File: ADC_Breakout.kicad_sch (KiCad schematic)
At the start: 36 parts, among them J0 Conn_01x06, J10 Conn_01x02, J11 Conn_01x02, J12 Conn_01x02, J13 Conn_01x02, J2 Digital Power, J3 Clock Chooser, J4 Analog Power, J6 Conn_01x02, J7 Conn_01x02, J8 Conn_01x02, J9 Conn_01x02, SW1 SW_MEC_5E, U2 SN74AUP2G80DCUR, X1 SIT8924BA-22-33E-8.192000, Y1 Crystal_Small

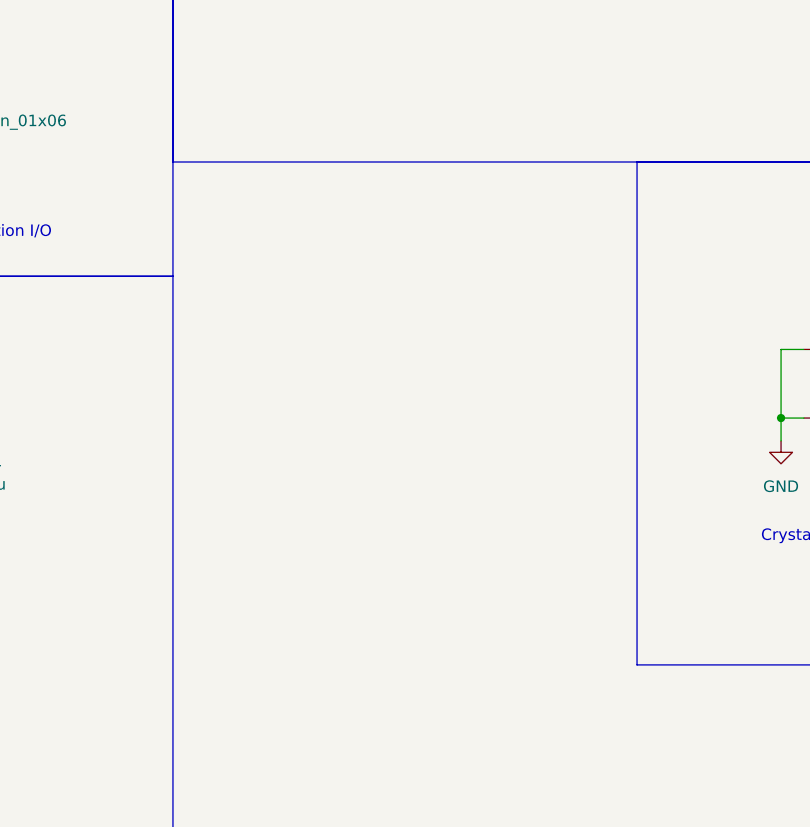
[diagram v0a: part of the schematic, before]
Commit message: Added graphics + iBOM
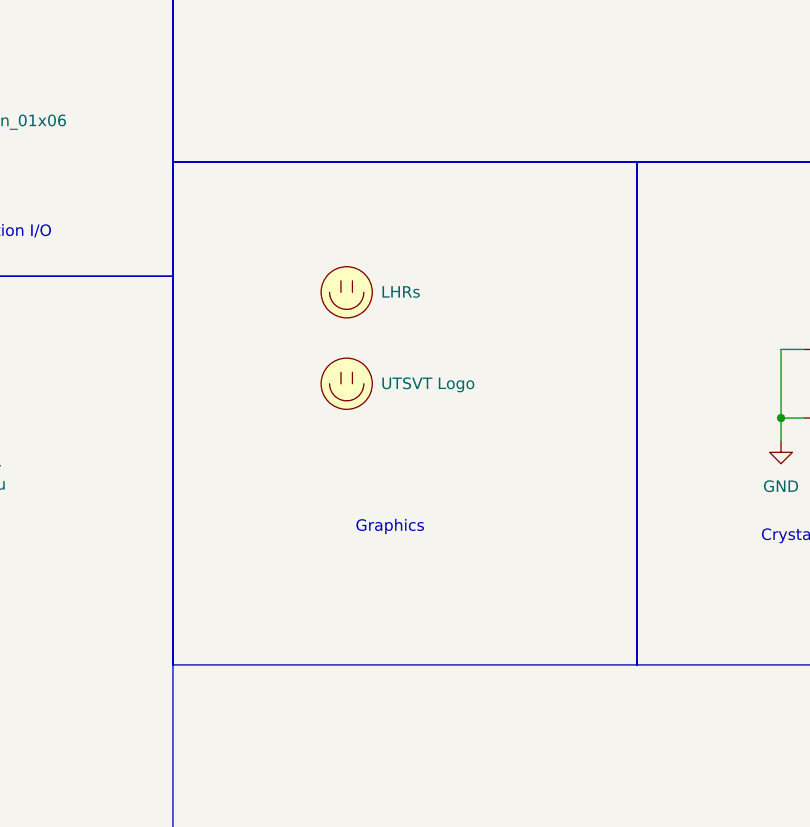
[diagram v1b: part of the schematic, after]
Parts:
- added LOGO0: LHRs, Top:LHRs_LOGO, symbol UTSVT_Misc:Logo_Placeholder
- added LOGO1: UTSVT Logo, SVT_Special:UTSVT_Logo_Symbol, symbol UTSVT_Misc:Logo_Placeholder
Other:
- note added: "Graphics"
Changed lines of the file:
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@@
 	)
 	(rectangle
+		(start 125.476 109.982)
+		(end 177.038 165.862)
+		(stroke
+			(width 0)
+			(type default)
+		)
+		(fill
+			(type none)
+		)
+	)
+	(rectangle
 		(start 11.938 122.682)
 		(end 125.476 198.12)
@@
 		)
 	)
+	(text "Graphics"
+		(exclude_from_sim no)
+		(at 149.606 150.622 0)
+		(effects
+			(font
+				(size 1.27 1.27)
+			)
+		)
+	)
 	(text "External Oscillator\nChosen from TI Development Board"
 		(exclude_from_sim no)
@@
 	)
 	(symbol
+		(lib_id "UTSVT_Misc:Logo_Placeholder")
+		(at 144.78 124.46 0)
+		(unit 1)
+		(exclude_from_sim no)
+		(in_bom yes)
+		(on_board yes)
+		(dnp no)
+		(fields_autoplaced yes)
+		(property "Reference" "LOGO0"
+			(at 144.78 120.65 0)
+			(effects
+				(font
+					(size 1.27 1.27)
+				)
+				(hide yes)
+			)
+		)
+		(property "Value" "LHRs"
+			(at 148.59 124.4599 0)
+			(effects
+				(font
+					(size 1.27 1.27)
+				)
+				(justify left)
+			)
+		)
+		(property "Footprint" "Top:LHRs_LOGO"
+			(at 144.78 122.555 0)
+			(effects
+				(font
+					(size 1.27 1.27)
+				)
+				(hide yes)
+			)
+		)
+		(property "Datasheet" ""
+			(at 144.78 122.555 0)
+			(effects
+				(font
+					(size 1.27 1.27)
+				)
+				(hide yes)
+			)
+		)
+		(property "Description" "Graph footprint placeholder"
+			(at 144.78 124.46 0)
+			(effects
+				(font
+					(size 1.27 1.27)
+				)
+				(hide yes)
+			)
+		)
+		(instances
+			(project ""
+				(path "/9e6f337e-b8cc-44e4-808a-ba1b350193a1"
+					(reference "LOGO0")
+					(unit 1)
+				)
+			)
+		)
+	)
+	(symbol
 		(lib_id "power:GND")
 		(at 236.22 52.07 0)
@@
 					(unit 1)
 				)
+			)
+		)
+	)
+	(symbol
+		(lib_id "UTSVT_Misc:Logo_Placeholder")
+		(at 144.78 134.62 0)
+		(unit 1)
+		(exclude_from_sim no)
+		(in_bom yes)
+		(on_board yes)
+		(dnp no)
+		(fields_autoplaced yes)
+		(property "Reference" "LOGO1"
+			(at 144.78 130.81 0)
+			(effects
+				(font
+					(size 1.27 1.27)
+				)
+				(hide yes)
+			)
+		)
+		(property "Value" "UTSVT Logo"
+			(at 148.59 134.6199 0)
+			(effects
+				(font
+					(size 1.27 1.27)
+				)
+				(justify left)
+			)
+		)
+		(property "Footprint" "SVT_Special:UTSVT_Logo_Symbol"
+			(at 144.78 132.715 0)
+			(effects
+				(font
+					(size 1.27 1.27)
+				)
+				(hide yes)
+			)
+		)
+		(property "Datasheet" ""
+			(at 144.78 132.715 0)
+			(effects
+				(font
+					(size 1.27 1.27)
+				)
+				(hide yes)
+			)
+		)
+		(property "Description" "Graph footprint placeholder"
+			(at 144.78 134.62 0)
+			(effects
+				(font
+					(size 1.27 1.27)
+				)
+				(hide yes)
+			)
+		)
+		(instances
+			(project "ADC_Breakout"
+				(path "/9e6f337e-b8cc-44e4-808a-ba1b350193a1"
+					(reference "LOGO1")
+					(unit 1)
+				)
